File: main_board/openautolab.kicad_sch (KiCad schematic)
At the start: 35 parts, among them J1 PIN11, J10 HX711, J11 LCD, J16 PWR_IN, J17 FILTER_PUMP, J18 FILTER_SENSOR, J2 PIN9, J3 PIN10, J4 PIN12, J6 PIN7, J7 PIN8, J8 PUMP, J9 SERVO, K1 FINDER-36.11, K2 FINDER-36.11, SW0 PIN_A0, SW1 PIN_A1, SW2 PIN_A2, SW3 SW_DPST_x2, SW4 SW_DPST_x2, U1 TD62064APG, U2 TD62064APG, U3 LM2576T-5

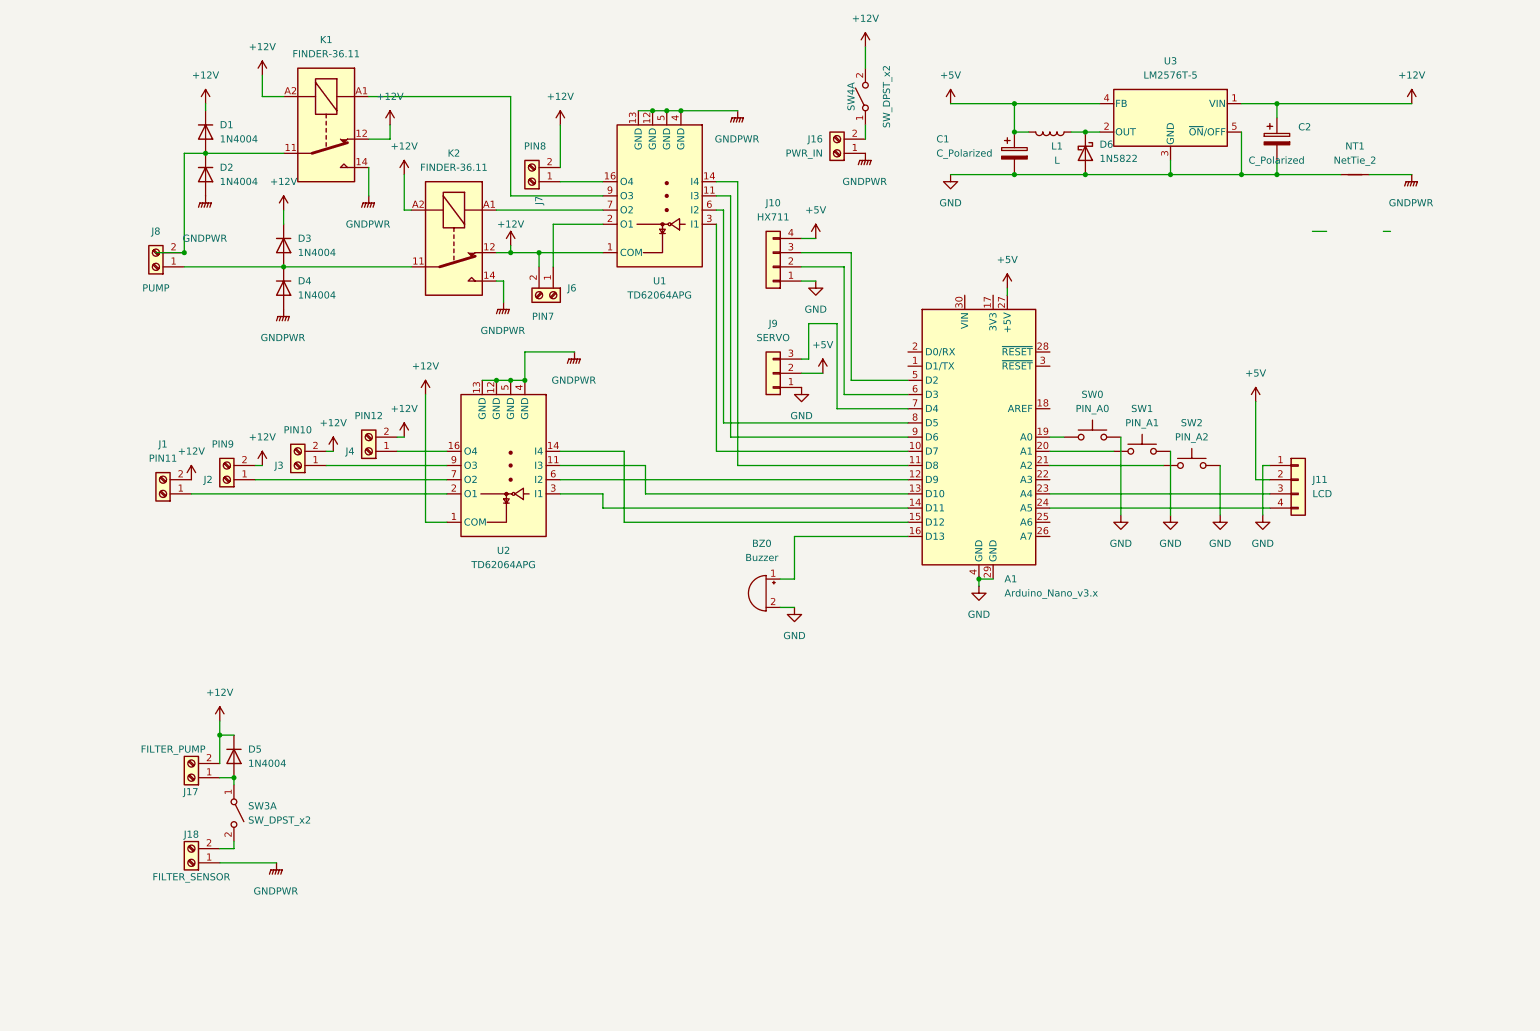
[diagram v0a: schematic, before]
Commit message: update board
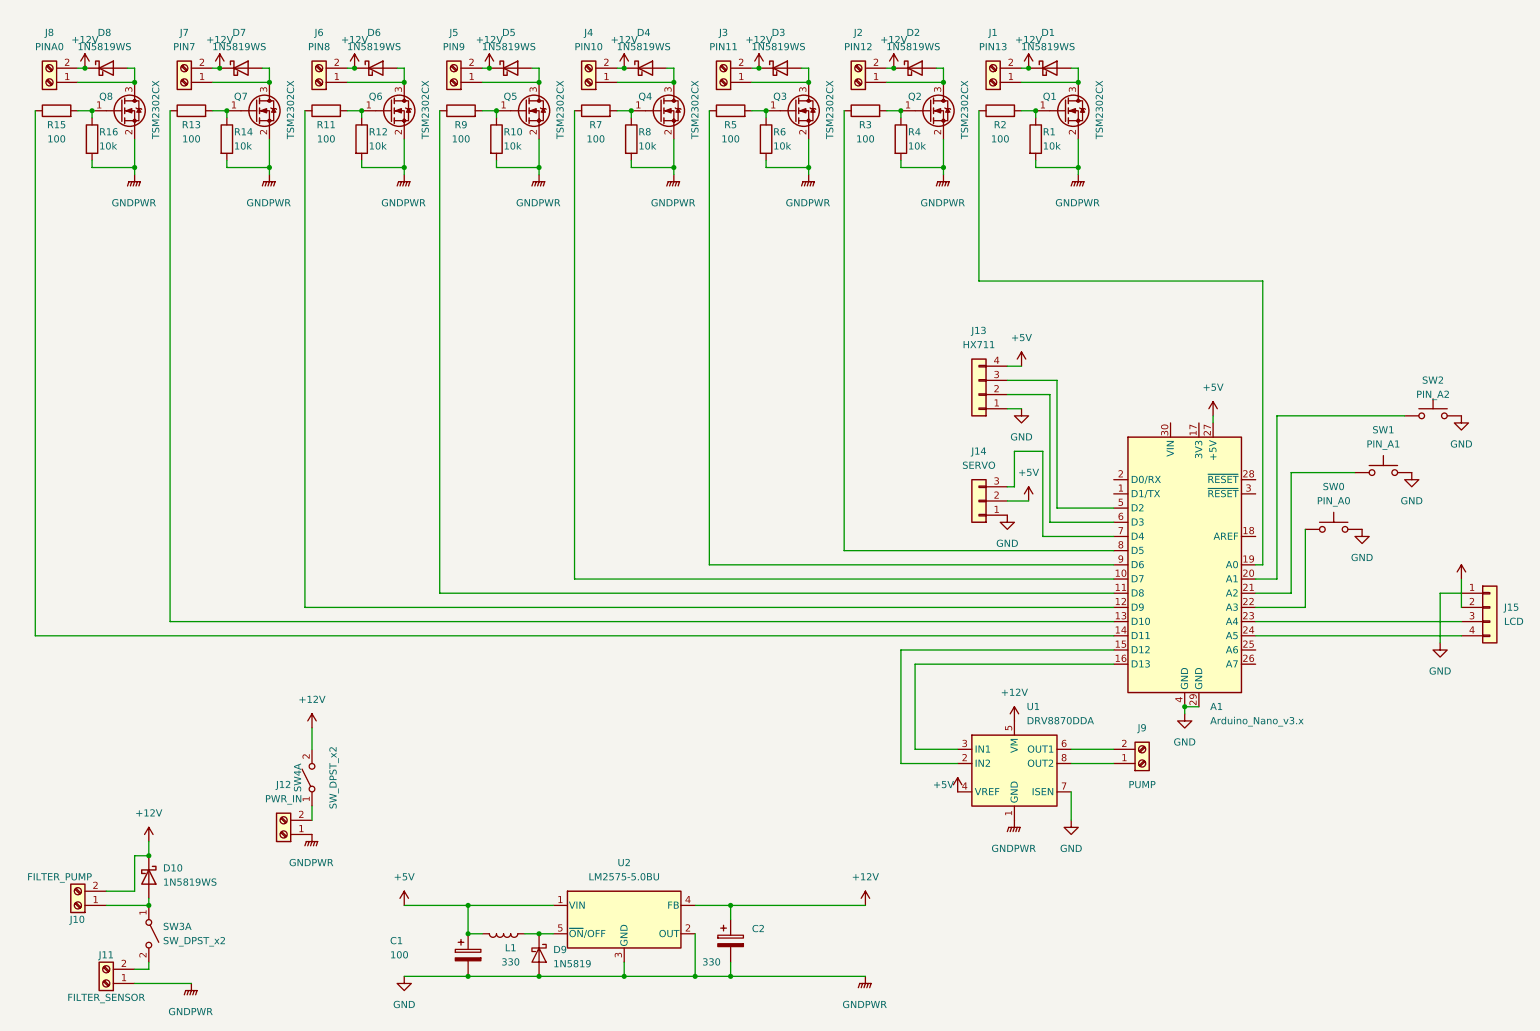
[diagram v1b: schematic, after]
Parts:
- removed BZ0: Buzzer, Buzzer_Beeper:Buzzer_12x9.5RM7.6, symbol Device:Buzzer
- removed D1, D2, D3, D4, D5: 1N4004, Diode_THT:D_DO-41_SOD81_P10.16mm_Horizontal, symbol Diode:1N4004
- removed D6: 1N5822, Diode_THT:D_DO-201AD_P15.24mm_Horizontal, symbol Diode:1N5822
- removed K1, K2: FINDER-36.11, Relay_THT:Relay_SPDT_Finder_36.11, symbol Relay:FINDER-36.11
- removed NT1: NetTie_2, NetTie:NetTie-2_SMD_Pad2.0mm, symbol Device:NetTie_2
- removed U1, U2: TD62064APG, Package_DIP:DIP-16_W7.62mm, symbol Transistor_Array:TD62064APG
- removed U3: LM2576T-5, Package_TO_SOT_THT:TO-220-5_Vertical, symbol Regulator_Switching:LM2576T-5
- added D1, D10, D2, D3, D4, D5, D6, D7, D8: 1N5819WS, Diode_SMD:D_SOD-323, symbol Diode:1N5819WS
- added D9: 1N5819, Diode_SMD:D_SOD-323, symbol Diode:1N5819
- added J5: PIN9, TerminalBlock_Phoenix:TerminalBlock_Phoenix_PT-1,5-2-3.5-H_1x02_P3.50mm_Horizontal, symbol Connector:Screw_Terminal_01x02
- added J9: PUMP, TerminalBlock_Phoenix:TerminalBlock_Phoenix_MKDS-3-2-5.08_1x02_P5.08mm_Horizontal, symbol Connector:Screw_Terminal_01x02
- added Q1, Q2, Q3, Q4, Q5, Q6, Q7, Q8: TSM2302CX, Package_TO_SOT_SMD:SOT-23, symbol Transistor_FET:TSM2302CX
- added R1, R10, R12, R14, R16, R4, R6, R8: 10k, Resistor_SMD:R_0603_1608Metric, symbol Device:R
- added R11, R13, R15, R2, R3, R5, R7, R9: 100, Resistor_SMD:R_0603_1608Metric, symbol Device:R
- added U1: DRV8870DDA, Package_SO:Texas_HTSOP-8-1EP_3.9x4.9mm_P1.27mm_EP2.95x4.9mm_Mask2.4x3.1mm_ThermalVias, symbol Driver_Motor:DRV8870DDA
- added U2: LM2575-5.0BU, Package_TO_SOT_SMD:TO-263-5_TabPin3, symbol Regulator_Switching:LM2575-5.0BU
- C1: value C_Polarized -> 100; footprint Capacitor_THT:CP_Radial_D10.0mm_P5.00mm -> Capacitor_SMD:CP_Elec_6.3x5.4
- C2: value C_Polarized -> 330; footprint Capacitor_THT:CP_Radial_D8.0mm_P5.00mm -> Capacitor_SMD:CP_Elec_8x10
- J1: value PIN11 -> PIN13; footprint TerminalBlock_Phoenix:TerminalBlock_Phoenix_MKDS-3-2-5.08_1x02_P5.08mm_Horizontal -> TerminalBlock_Phoenix:TerminalBlock_Phoenix_PT-1,5-2-3.5-H_1x02_P3.50mm_Horizontal
- J2: value PIN9 -> PIN12; footprint TerminalBlock_Phoenix:TerminalBlock_Phoenix_MKDS-3-2-5.08_1x02_P5.08mm_Horizontal -> TerminalBlock_Phoenix:TerminalBlock_Phoenix_PT-1,5-2-3.5-H_1x02_P3.50mm_Horizontal
- J3: value PIN10 -> PIN11; footprint TerminalBlock_Phoenix:TerminalBlock_Phoenix_MKDS-3-2-5.08_1x02_P5.08mm_Horizontal -> TerminalBlock_Phoenix:TerminalBlock_Phoenix_PT-1,5-2-3.5-H_1x02_P3.50mm_Horizontal
- J4: value PIN12 -> PIN10; footprint TerminalBlock_Phoenix:TerminalBlock_Phoenix_MKDS-3-2-5.08_1x02_P5.08mm_Horizontal -> TerminalBlock_Phoenix:TerminalBlock_Phoenix_PT-1,5-2-3.5-H_1x02_P3.50mm_Horizontal
- J6: value PIN7 -> PIN8; footprint TerminalBlock_Phoenix:TerminalBlock_Phoenix_MKDS-3-2-5.08_1x02_P5.08mm_Horizontal -> TerminalBlock_Phoenix:TerminalBlock_Phoenix_PT-1,5-2-3.5-H_1x02_P3.50mm_Horizontal
- J7: value PIN8 -> PIN7; footprint TerminalBlock_Phoenix:TerminalBlock_Phoenix_MKDS-3-2-5.08_1x02_P5.08mm_Horizontal -> TerminalBlock_Phoenix:TerminalBlock_Phoenix_PT-1,5-2-3.5-H_1x02_P3.50mm_Horizontal
- J8: value PUMP -> PINA0; footprint TerminalBlock_Phoenix:TerminalBlock_Phoenix_MKDS-3-2-5.08_1x02_P5.08mm_Horizontal -> TerminalBlock_Phoenix:TerminalBlock_Phoenix_PT-1,5-2-3.5-H_1x02_P3.50mm_Horizontal
- L1: value L -> 330; footprint Inductor_THT:L_Toroid_Vertical_L26.7mm_W14.0mm_P10.16mm_Pulse_D -> Inductor_SMD:L_12x12mm_H8mm
- SW0, SW1, SW2: footprint Button_Switch_THT:SW_PUSH_6mm -> Button_Switch_SMD:SW_Push_1P1T_NO_6x6mm_H9.5mm
- renumbered J17 to J10, J18 to J11, J16 to J12, J10 to J13, J9 to J14, J11 to J15
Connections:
- net GNDPWR is gone; now on net GND: J11.1 (Pin_1), J12.1 (Pin_1)
- net +12V: now also J8.2 (Pin_2), D1.1 (K), D10.1 (K), D2.1 (K), D3.1 (K), D4.1 (K), D5.1 (K), D6.1 (K), D7.1 (K), D8.1 (K), J5.2 (Pin_2), U1.5 (VM), U2.4 (FB)
- net +5V: now also U1.4 (VREF), U2.1 (VIN)
- net GND: now also D9.2 (A), Q1.2 (S), Q2.2 (S), Q3.2 (S), Q4.2 (S), Q5.2 (S), Q6.2 (S), Q7.2 (S), Q8.2 (S), R1.2, R10.2, R12.2, R14.2, R16.2, R4.2, R6.2, R8.2, U1.1 (GND), U1.7 (ISEN), U1.9 (GND), U2.2 (OUT), U2.3 (GND)
- net at J8.1 (Pin_1): now also D8.2 (A), Q8.3 (D)
- net at J4.1 (Pin_1): now also D4.2 (A), Q4.3 (D)
- net at J3.1 (Pin_1): now also D3.2 (A), Q3.3 (D)
- net at J7.1 (Pin_1): now also D7.2 (A), Q7.3 (D)
- net at SW1.1: now also A1.21 (A2); no longer A1.20 (A1)
- net at J2.1 (Pin_1): now also D2.2 (A), Q2.3 (D)
- net at A1.9 (D6): now also R5.1
- net at A1.11 (D8): now also R9.1
- net at J6.1 (Pin_1): now also D6.2 (A), Q6.3 (D)
- net at A1.10 (D7): now also R7.1
- net at A1.8 (D5): now also R3.1
- net at L1.1: now also D9.1 (K), U2.5 (~{ON}/OFF)
- net at A1.13 (D10): now also R13.1
- net at A1.15 (D12): now also U1.2 (IN2)
- net at J1.1 (Pin_1): now also D1.2 (A), Q1.3 (D)
- net at A1.14 (D11): now also R15.1
- net at A1.12 (D9): now also R11.1
- net at J10.1 (Pin_1), SW3.1 (A): now also D10.2 (A)
- net at A1.19 (A0): now also R2.1; no longer SW0.1
- net at SW2.1: now also A1.20 (A1); no longer A1.21 (A2)
- net at A1.16 (D13): now also U1.3 (IN1)
- net at A1.22 (A3): now also SW0.1
- new net: Q6.1 (G), R11.2, R12.1
- new net: J9.1 (Pin_1), U1.8 (OUT2)
- new net: J9.2 (Pin_2), U1.6 (OUT1)
- new net: D5.2 (A), J5.1 (Pin_1), Q5.3 (D)
- new net: Q8.1 (G), R15.2, R16.1
- new net: Q5.1 (G), R10.1, R9.2
- new net: Q1.1 (G), R1.1, R2.2
- new net: Q3.1 (G), R5.2, R6.1
- new net: Q7.1 (G), R13.2, R14.1
- new net: Q4.1 (G), R7.2, R8.1
- new net: Q2.1 (G), R3.2, R4.1
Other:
- moved on the sheet: A1, C1, C2, J1, J10, J11, J12, J13, J14, J15, L1, SW0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

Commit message: update schematic, complete parts description
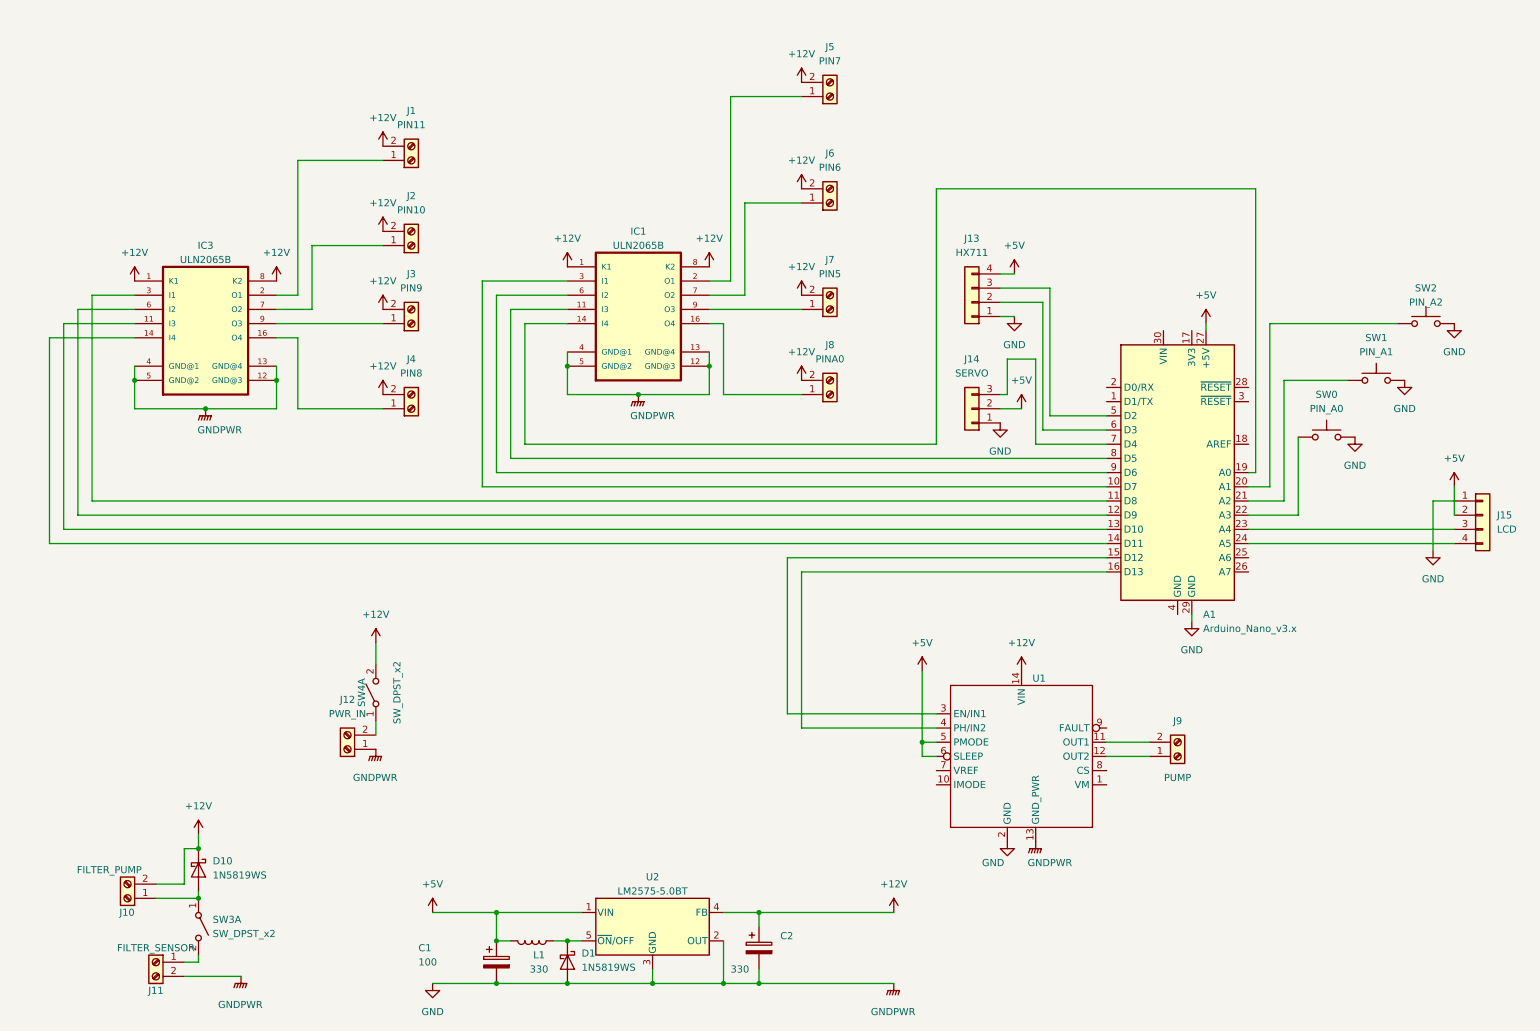
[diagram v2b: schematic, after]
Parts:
- removed D1, D2, D3, D4, D5, D6, D7, D8: 1N5819WS, Diode_SMD:D_SOD-323, symbol Diode:1N5819WS
- removed D9: 1N5819, Diode_SMD:D_SOD-323, symbol Diode:1N5819
- removed Q1, Q2, Q3, Q4, Q5, Q6, Q7, Q8: TSM2302CX, Package_TO_SOT_SMD:SOT-23, symbol Transistor_FET:TSM2302CX
- removed R1, R10, R12, R14, R16, R4, R6, R8: 10k, Resistor_SMD:R_0603_1608Metric, symbol Device:R
- removed R11, R13, R15, R2, R3, R5, R7, R9: 100, Resistor_SMD:R_0603_1608Metric, symbol Device:R
- removed U1: DRV8870DDA, Package_SO:Texas_HTSOP-8-1EP_3.9x4.9mm_P1.27mm_EP2.95x4.9mm_Mask2.4x3.1mm_ThermalVias, symbol Driver_Motor:DRV8870DDA
- removed U2: LM2575-5.0BU, Package_TO_SOT_SMD:TO-263-5_TabPin3, symbol Regulator_Switching:LM2575-5.0BU
- added D1: 1N5819WS, Diode_THT:D_A-405_P7.62mm_Horizontal, symbol Device:D_Schottky
- added IC1, IC3: ULN2065B, Package_DIP:DIP-16_W7.62mm, symbol ULN2065B:ULN2065B
- added U1: ~, Pololu_breakout_DRV8874:Pololu_breakout_DRV8874, symbol Pololu_breakout_DRV8874:Pololu_breakout_DRV8874
- added U2: LM2575-5.0BT, Package_TO_SOT_THT:TO-220-5_P3.4x3.7mm_StaggerOdd_Lead3.8mm_Vertical, symbol Regulator_Switching:LM2575-5.0BT
- C1: footprint Capacitor_SMD:CP_Elec_6.3x5.4 -> Capacitor_THT:CP_Radial_D8.0mm_P5.00mm
- C2: footprint Capacitor_SMD:CP_Elec_8x10 -> Capacitor_THT:CP_Radial_D8.0mm_P5.00mm
- D10: footprint Diode_SMD:D_SOD-323 -> Diode_THT:D_A-405_P7.62mm_Horizontal; symbol Diode:1N5819WS -> Device:D_Schottky
- J1: value PIN13 -> PIN11
- J2: value PIN12 -> PIN10
- J3: value PIN11 -> PIN9
- J4: value PIN10 -> PIN8
- J5: value PIN9 -> PIN7
- J6: value PIN8 -> PIN6
- J7: value PIN7 -> PIN5
- L1: footprint Inductor_SMD:L_12x12mm_H8mm -> Inductor_THT:L_Radial_D12.0mm_P5.00mm_Fastron_11P
- SW0, SW1, SW2: footprint Button_Switch_SMD:SW_Push_1P1T_NO_6x6mm_H9.5mm -> Button_Switch_THT:SW_PUSH_6mm
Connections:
- net +12V: now also IC1.1 (K1), IC1.8 (K2), IC3.1 (K1), IC3.8 (K2), U1.14 (VIN), U2.4 (FB)
- net +5V: now also U1.5 (PMODE), U1.6 (SLEEP), U2.1 (VIN)
- net GND: now also J11.2 (Pin_2), D1.2 (A), IC1.12 (GND@3), IC1.13 (GND@4), IC1.4 (GND@1), IC1.5 (GND@2), IC3.12 (GND@3), IC3.13 (GND@4), IC3.4 (GND@1), IC3.5 (GND@2), U1.13 (GND_PWR), U1.2 (GND), U2.2 (OUT), U2.3 (GND); no longer A1.4 (GND), J11.1 (Pin_1)
- net at J6.1 (Pin_1): now also IC1.7 (O2)
- net at J9.1 (Pin_1): now also U1.12 (OUT2)
- net at J9.2 (Pin_2): now also U1.11 (OUT1)
- net at J4.1 (Pin_1): now also IC3.16 (O4)
- net at J5.1 (Pin_1): now also IC1.2 (O1)
- net at J8.1 (Pin_1): now also IC1.16 (O4)
- net at A1.11 (D8): now also IC3.3 (I1)
- net at A1.19 (A0): now also IC1.14 (I4)
- net at SW3.2 (B): now also J11.1 (Pin_1); no longer J11.2 (Pin_2)
- net at A1.13 (D10): now also IC3.11 (I3)
- net at J3.1 (Pin_1): now also IC3.9 (O3)
- net at A1.14 (D11): now also IC3.14 (I4)
- net at J1.1 (Pin_1): now also IC3.2 (O1)
- net at J2.1 (Pin_1): now also IC3.7 (O2)
- net at J7.1 (Pin_1): now also IC1.9 (O3)
- net at A1.10 (D7): now also IC1.3 (I1)
- net at A1.12 (D9): now also IC3.6 (I2)
- net at A1.15 (D12): now also U1.3 (EN/IN1)
- net at A1.16 (D13): now also U1.4 (PH/IN2)
- net at A1.8 (D5): now also IC1.11 (I3)
- net at A1.9 (D6): now also IC1.6 (I2)
- net at L1.1: now also D1.1 (K), U2.5 (~{ON}/OFF)
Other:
- moved on the sheet: A1, C1, C2, D10, J10, J11, J12, J13, J14, J15, J9, L1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
